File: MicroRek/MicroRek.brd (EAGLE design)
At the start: 40 x 30 mm, 18 parts, among them IC3 LSM9DS1TR

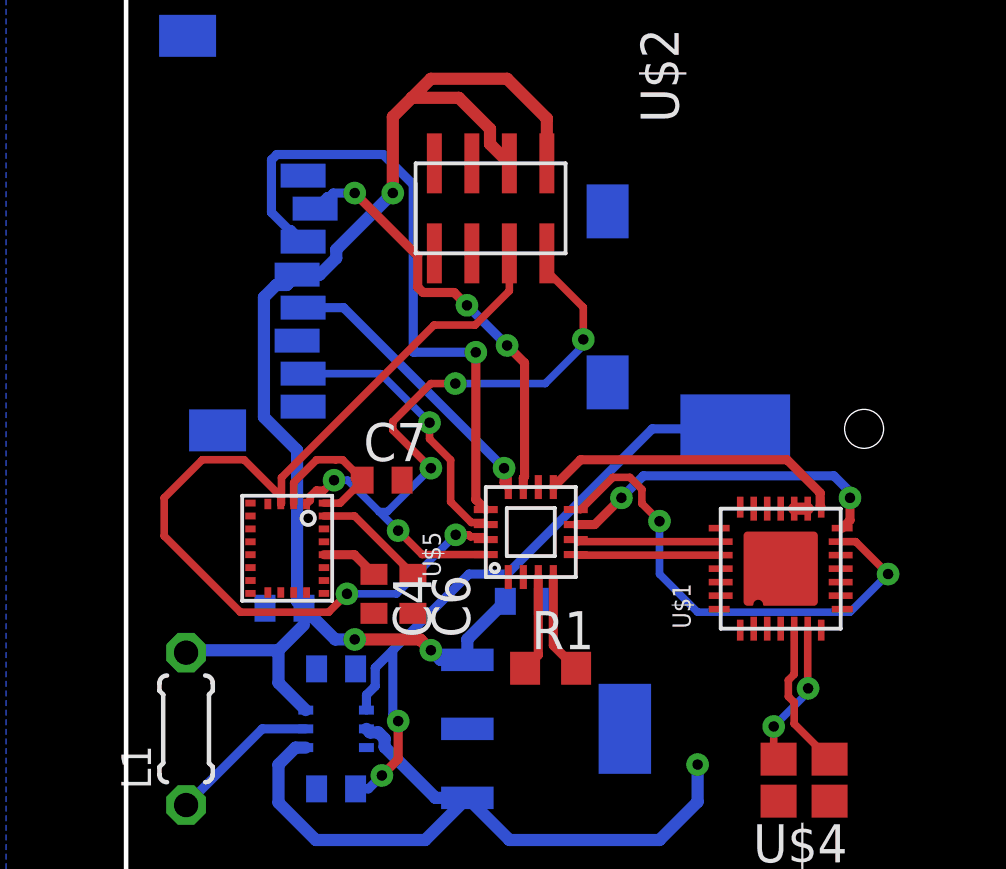
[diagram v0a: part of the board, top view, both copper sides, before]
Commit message: updated board layout
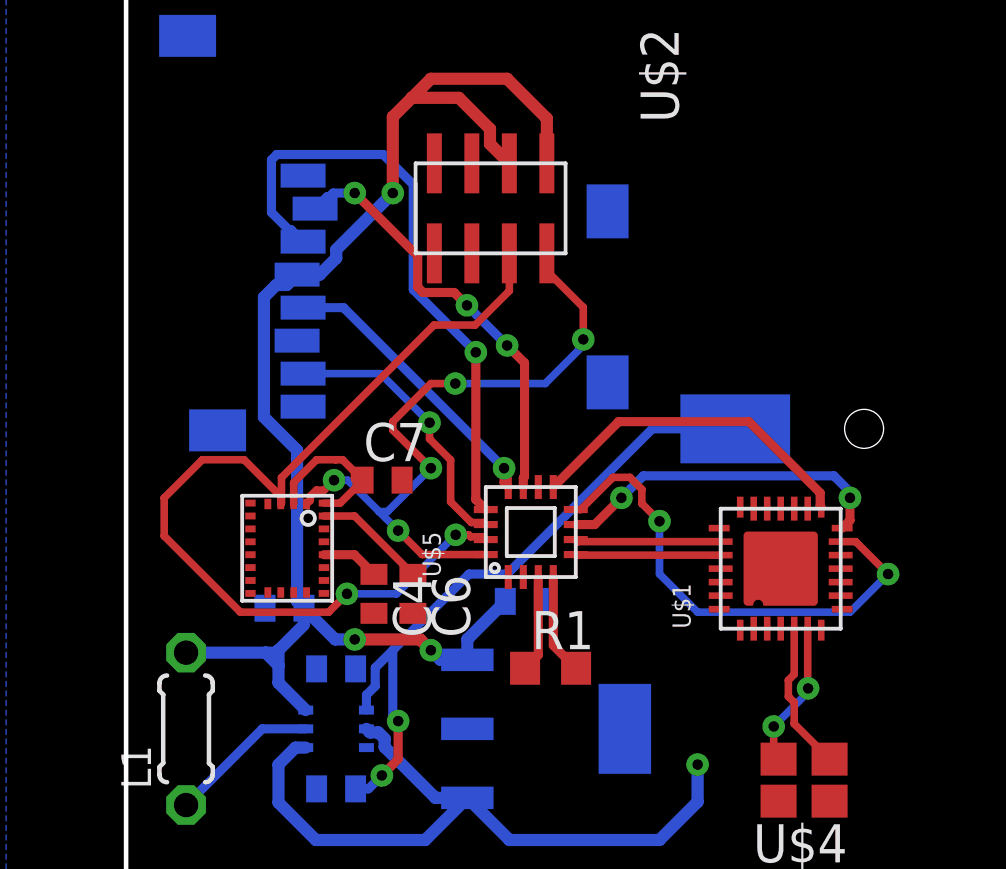
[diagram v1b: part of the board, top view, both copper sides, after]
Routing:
- net MOSI3: track 21.5 -> 20.3 mm
- net SCK5: track 10.2 -> 11.3 mm
- net 3.3V: track 47.4 -> 48.0 mm
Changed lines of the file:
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@@
 <wire x1="8.6171" y1="4.67229375" x2="8.6171" y2="4.3944" width="0.4064" layer="16"/>
 <wire x1="8.6171" y1="4.3944" x2="10.3115" y2="2.7" width="0.4064" layer="16"/>
-<wire x1="22.72" y1="12.34" x2="22.27" y2="12.34" width="0.4064" layer="1"/>
+<wire x1="22.27" y1="12.34" x2="22.72" y2="12.34" width="0" layer="19" extent="1-16"/>
 <wire x1="11.375" y1="2.7" x2="9.9704" y2="1.2954" width="0.4064" layer="16"/>
 <wire x1="6.3246" y1="1.2954" x2="5.08" y2="2.54" width="0.4064" layer="16"/>
@@
 <contactref element="U$5" pad="P8"/>
 <contactref element="U$1" pad="P15"/>
-<wire x1="23.17" y1="12.39" x2="23.1348" y2="12.4252" width="0.3048" layer="1"/>
-<wire x1="23.1348" y1="12.4252" x2="23.1348" y2="12.86625" width="0.3048" layer="1"/>
-<wire x1="23.1348" y1="12.86625" x2="22.03105" y2="13.97" width="0.3048" layer="1"/>
-<wire x1="15.15" y1="13.97" x2="14.24" y2="13.06" width="0.3048" layer="1"/>
-<wire x1="22.03105" y1="13.97" x2="15.15" y2="13.97" width="0.3048" layer="1"/>
+<wire x1="14.24" y1="13.06" x2="16.42" y2="15.24" width="0.3048" layer="1"/>
+<wire x1="23.1348" y1="12.86625" x2="23.1348" y2="12.4252" width="0.3048" layer="1"/>
+<wire x1="23.1348" y1="12.4252" x2="23.17" y2="12.39" width="0.3048" layer="1"/>
+<wire x1="16.42" y1="15.24" x2="20.76105" y2="15.24" width="0.3048" layer="1"/>
+<wire x1="20.76105" y1="15.24" x2="23.1348" y2="12.86625" width="0.3048" layer="1"/>
 </signal>
 <signal name="MISO3">
@@
 <wire x1="11.65749375" y1="12.64250625" x2="11.65749375" y2="17.55250625" width="0.3048" layer="1"/>
 <via x="11.65749375" y="17.55250625" extent="1-16" drill="0.35"/>
-<wire x1="11.65749375" y1="17.55250625" x2="9.58749375" y2="17.55250625" width="0.3048" layer="16"/>
 <wire x1="5.02375" y1="24.1448" x2="4.8452" y2="23.96625" width="0.3048" layer="16"/>
-<wire x1="9.58749375" y1="17.55250625" x2="9.573" y2="17.567" width="0.3048" layer="16"/>
 <wire x1="5.42375" y1="21.6352" x2="5.5048" y2="21.6352" width="0.3048" layer="16"/>
 <wire x1="5.5048" y1="21.6352" x2="5.9" y2="21.24" width="0.3048" layer="16"/>
-<wire x1="9.573" y1="17.567" x2="9.573" y2="23.1429125" width="0.3048" layer="16"/>
 <wire x1="4.8452" y1="23.96625" x2="4.8452" y2="22.21375" width="0.3048" layer="16"/>
 <wire x1="4.8452" y1="22.21375" x2="5.42375" y2="21.6352" width="0.3048" layer="16"/>
 <wire x1="9.573" y1="23.1429125" x2="8.5711125" y2="24.1448" width="0.3048" layer="16"/>
 <wire x1="8.5711125" y1="24.1448" x2="5.02375" y2="24.1448" width="0.3048" layer="16"/>
+<wire x1="11.65749375" y1="17.55250625" x2="9.573" y2="19.637" width="0.3048" layer="16"/>
+<wire x1="9.573" y1="19.637" x2="9.573" y2="23.1429125" width="0.3048" layer="16"/>
 </signal>
 <signal name="SCK3">
@@
 <wire x1="12.1306" y1="24.99729375" x2="11.09289375" y2="26.035" width="0.4064" layer="1"/>
 <wire x1="11.09289375" y1="26.035" x2="9.525" y2="26.035" width="0.4064" layer="1"/>
-<wire x1="2" y1="7.54" x2="2.08" y2="7.62" width="0.3048" layer="16"/>
-<wire x1="2.08" y1="7.62" x2="5.08" y2="7.62" width="0.4064" layer="16"/>
 <wire x1="5.08" y1="7.62" x2="5.93" y2="8.47" width="0.4064" layer="16"/>
 <wire x1="5.93" y1="8.47" x2="5.93" y2="9.02" width="0.3048" layer="16"/>
@@
 <wire x1="4.5944" y1="19.38729375" x2="4.5944" y2="15.39270625" width="0.4064" layer="16"/>
 <wire x1="4.5944" y1="15.39270625" x2="5.7" y2="14.28710625" width="0.4064" layer="16"/>
-<wire x1="5.08" y1="7.62" x2="5.08" y2="6.5335" width="0.4064" layer="16"/>
+<wire x1="5.08" y1="7.62" x2="5.08" y2="7.112" width="0.4064" layer="16"/>
+<wire x1="5.08" y1="7.112" x2="5.08" y2="6.5335" width="0.4064" layer="16"/>
 <wire x1="5.08" y1="6.5335" x2="5.9885" y2="5.625" width="0.4064" layer="16"/>
 <wire x1="11.375" y1="7.3" x2="10.48" y2="7.3" width="0.4064" layer="16"/>
@@
 <wire x1="10.16" y1="7.62" x2="9.7994" y2="7.9806" width="0.4064" layer="1"/>
 <wire x1="9.7994" y1="7.9806" x2="7.62" y2="7.9806" width="0.4064" layer="1"/>
+<wire x1="2" y1="7.54" x2="4.652" y2="7.54" width="0.4064" layer="16"/>
+<wire x1="4.652" y1="7.54" x2="5.08" y2="7.112" width="0.4064" layer="16"/>
+<wire x1="4.652" y1="7.54" x2="5" y2="7.54" width="0.4064" layer="16"/>
+<wire x1="5" y1="7.54" x2="5.08" y2="7.62" width="0.4064" layer="16"/>
 </signal>
 <signal name="N$7">
